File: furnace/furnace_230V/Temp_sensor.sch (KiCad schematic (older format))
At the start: 1 part

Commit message: Add files via upload
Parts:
- added C?: 0,1, Capacitor_SMD:C_0603_1608Metric_Pad1.08x0.95mm_HandSolder, symbol Device:C
- added R?: 4,7k, Resistor_SMD:R_0603_1608Metric_Pad0.98x0.95mm_HandSolder, symbol Device:R
- added TP?: TestPoint, symbol Connector:TestPoint
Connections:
- net labels added: +3V3, GND, SDA
- wire segments 0 -> 14
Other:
- note added: "1-wire temperature sensor"
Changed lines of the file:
@@
 L Sensor_Temperature:DS18B20 U?
 U 1 1 60AB486E
-P 5950 3550
-F 0 "U?" H 5720 3596 50  0000 R CNN
-F 1 "DS18B20" H 5720 3505 50  0000 R CNN
-F 2 "Package_TO_SOT_THT:TO-92_Inline" H 4950 3300 50  0001 C CNN
-F 3 "http://datasheets.maximintegrated.com/en/ds/DS18B20.pdf" H 5800 3800 50  0001 C CNN
-	1    5950 3550
+P 5500 4300
+F 0 "U?" H 5850 4650 50  0000 R CNN
+F 1 "DS18B20" H 6000 4550 50  0000 R CNN
+F 2 "Package_TO_SOT_THT:TO-92_Inline" H 4500 4050 50  0001 C CNN
+F 3 "http://datasheets.maximintegrated.com/en/ds/DS18B20.pdf" H 5350 4550 50  0001 C CNN
+	1    5500 4300
 	1    0    0    -1
 $EndComp
+$Comp
+L Device:C C?
+U 1 1 60AC6956
+P 5000 3650
+AR Path="/60AC6956" Ref="C?"  Part="1"
+AR Path="/609CA6A8/609D24C0/60AC6956" Ref="C?"  Part="1"
+AR Path="/609CA6A8/60A08E0B/60AC6956" Ref="C?"  Part="1"
+AR Path="/609CA6A8/60A0A46E/60AC6956" Ref="C?"  Part="1"
+AR Path="/609CA6A8/60A0A500/60AC6956" Ref="C?"  Part="1"
+AR Path="/609CA6A8/60A0A922/60AC6956" Ref="C?"  Part="1"
+AR Path="/609CA6A8/60AC6956" Ref="C?"  Part="1"
+AR Path="/609CA6A8/60AE5653/60AC6956" Ref="C?"  Part="1"
+AR Path="/60AAC605/60AC6956" Ref="C?"  Part="1"
+AR Path="/60AAE178/60AC6956" Ref="C?"  Part="1"
+F 0 "C?" H 5115 3696 50  0000 L CNN
+F 1 "0,1" H 5115 3605 50  0000 L CNN
+F 2 "Capacitor_SMD:C_0603_1608Metric_Pad1.08x0.95mm_HandSolder" H 5038 3500 50  0001 C CNN
+F 3 "~" H 5000 3650 50  0001 C CNN
+	1    5000 3650
+	1    0    0    -1
+$EndComp
+$Comp
+L Device:R R?
+U 1 1 60AC70EB
+P 6500 3650
+AR Path="/60AC70EB" Ref="R?"  Part="1"
+AR Path="/609CA6A8/60AC70EB" Ref="R?"  Part="1"
+AR Path="/609CA6A8/60AE5653/60AC70EB" Ref="R?"  Part="1"
+AR Path="/60AAC605/60AC70EB" Ref="R?"  Part="1"
+AR Path="/60AAE178/60AC70EB" Ref="R?"  Part="1"
+F 0 "R?" H 6570 3696 50  0000 L CNN
+F 1 "4,7k" H 6570 3605 50  0000 L CNN
+F 2 "Resistor_SMD:R_0603_1608Metric_Pad0.98x0.95mm_HandSolder" V 6430 3650 50  0001 C CNN
+F 3 "~" H 6500 3650 50  0001 C CNN
+	1    6500 3650
+	1    0    0    -1
+$EndComp
+$Comp
+L Connector:TestPoint TP?
+U 1 1 60ACF1AA
+P 7000 4500
+AR Path="/60ACF1AA" Ref="TP?"  Part="1"
+AR Path="/609CA6A8/60AE5653/60ACF1AA" Ref="TP?"  Part="1"
+AR Path="/60AAC605/60ACF1AA" Ref="TP?"  Part="1"
+AR Path="/60AAE178/60ACF1AA" Ref="TP?"  Part="1"
+F 0 "TP?" H 7058 4618 50  0000 L CNN
+F 1 "TestPoint" H 7058 4527 50  0001 L CNN
+F 2 "" H 7200 4500 50  0001 C CNN
+F 3 "~" H 7200 4500 50  0001 C CNN
+	1    7000 4500
+	1    0    0    -1
+$EndComp
+Text Notes 7950 2300 2    197  ~ 0
+1-wire temperature sensor
+Text HLabel 7500 4500 2    50   BiDi ~ 0
+SDA
+Text HLabel 4500 3500 0    50   Input ~ 0
++3V3
+Text HLabel 4500 5000 0    50   Input ~ 0
+GND
+Wire Wire Line
+	4500 3500 5000 3500
+Connection ~ 5000 3500
+Wire Wire Line
+	5000 3500 5500 3500
+Wire Wire Line
+	5500 4000 5500 3500
+Connection ~ 5500 3500
+Wire Wire Line
+	5500 3500 6500 3500
+Wire Wire Line
+	5000 3800 5000 5000
+Wire Wire Line
+	5000 5000 4500 5000
+Wire Wire Line
+	5500 4600 5500 5000
+Wire Wire Line
+	5500 5000 5000 5000
+Connection ~ 5000 5000
+Wire Wire Line
+	5800 4300 6000 4300
+Wire Wire Line
+	6000 4300 6000 4500
+Wire Wire Line
+	6000 4500 6500 4500
+Connection ~ 7000 4500
+Wire Wire Line
+	7000 4500 7500 4500
+Wire Wire Line
+	6500 3800 6500 4500
+Connection ~ 6500 4500
+Wire Wire Line
+	6500 4500 7000 4500
 $EndSCHEMATC

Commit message: Add files via upload
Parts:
- C14: renamed from C?; symbol Device:C -> furnace_230V-rescue:C-Device
- R9: renamed from R?; symbol Device:R -> furnace_230V-rescue:R-Device
- TP6: renamed from TP?; symbol Connector:TestPoint -> furnace_230V-rescue:TestPoint-Connector
- U4: renamed from U?; symbol Sensor_Temperature:DS18B20 -> furnace_230V-rescue:DS18B20-Sensor_Temperature
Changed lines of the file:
@@
 $EndDescr
 $Comp
-L Sensor_Temperature:DS18B20 U?
+L furnace_230V-rescue:DS18B20-Sensor_Temperature U4
 U 1 1 60AB486E
 P 5500 4300
-F 0 "U?" H 5850 4650 50  0000 R CNN
+F 0 "U4" H 5850 4650 50  0000 R CNN
 F 1 "DS18B20" H 6000 4550 50  0000 R CNN
 F 2 "Package_TO_SOT_THT:TO-92_Inline" H 4500 4050 50  0001 C CNN
@@
 $EndComp
 $Comp
-L Device:C C?
+L furnace_230V-rescue:C-Device C?
 U 1 1 60AC6956
 P 5000 3650
@@
 AR Path="/609CA6A8/60AE5653/60AC6956" Ref="C?"  Part="1"
 AR Path="/60AAC605/60AC6956" Ref="C?"  Part="1"
-AR Path="/60AAE178/60AC6956" Ref="C?"  Part="1"
-F 0 "C?" H 5115 3696 50  0000 L CNN
+AR Path="/60AAE178/60AC6956" Ref="C14"  Part="1"
+F 0 "C14" H 5115 3696 50  0000 L CNN
 F 1 "0,1" H 5115 3605 50  0000 L CNN
 F 2 "Capacitor_SMD:C_0603_1608Metric_Pad1.08x0.95mm_HandSolder" H 5038 3500 50  0001 C CNN
@@
 $EndComp
 $Comp
-L Device:R R?
+L furnace_230V-rescue:R-Device R?
 U 1 1 60AC70EB
 P 6500 3650
@@
 AR Path="/609CA6A8/60AE5653/60AC70EB" Ref="R?"  Part="1"
 AR Path="/60AAC605/60AC70EB" Ref="R?"  Part="1"
-AR Path="/60AAE178/60AC70EB" Ref="R?"  Part="1"
-F 0 "R?" H 6570 3696 50  0000 L CNN
+AR Path="/60AAE178/60AC70EB" Ref="R9"  Part="1"
+F 0 "R9" H 6570 3696 50  0000 L CNN
 F 1 "4,7k" H 6570 3605 50  0000 L CNN
 F 2 "Resistor_SMD:R_0603_1608Metric_Pad0.98x0.95mm_HandSolder" V 6430 3650 50  0001 C CNN
@@
 $EndComp
 $Comp
-L Connector:TestPoint TP?
+L furnace_230V-rescue:TestPoint-Connector TP?
 U 1 1 60ACF1AA
 P 7000 4500
@@
 AR Path="/609CA6A8/60AE5653/60ACF1AA" Ref="TP?"  Part="1"
 AR Path="/60AAC605/60ACF1AA" Ref="TP?"  Part="1"
-AR Path="/60AAE178/60ACF1AA" Ref="TP?"  Part="1"
-F 0 "TP?" H 7058 4618 50  0000 L CNN
+AR Path="/60AAE178/60ACF1AA" Ref="TP6"  Part="1"
+F 0 "TP6" H 7058 4618 50  0000 L CNN
 F 1 "TestPoint" H 7058 4527 50  0001 L CNN
 F 2 "" H 7200 4500 50  0001 C CNN

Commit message: Add files via upload
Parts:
- TP6: footprint (none) -> MountingHole:MountingHole_2.2mm_M2_DIN965_Pad_TopBottom
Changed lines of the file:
@@
 F 0 "TP6" H 7058 4618 50  0000 L CNN
 F 1 "TestPoint" H 7058 4527 50  0001 L CNN
-F 2 "" H 7200 4500 50  0001 C CNN
+F 2 "MountingHole:MountingHole_2.2mm_M2_DIN965_Pad_TopBottom" H 7200 4500 50  0001 C CNN
 F 3 "~" H 7200 4500 50  0001 C CNN
 	1    7000 4500

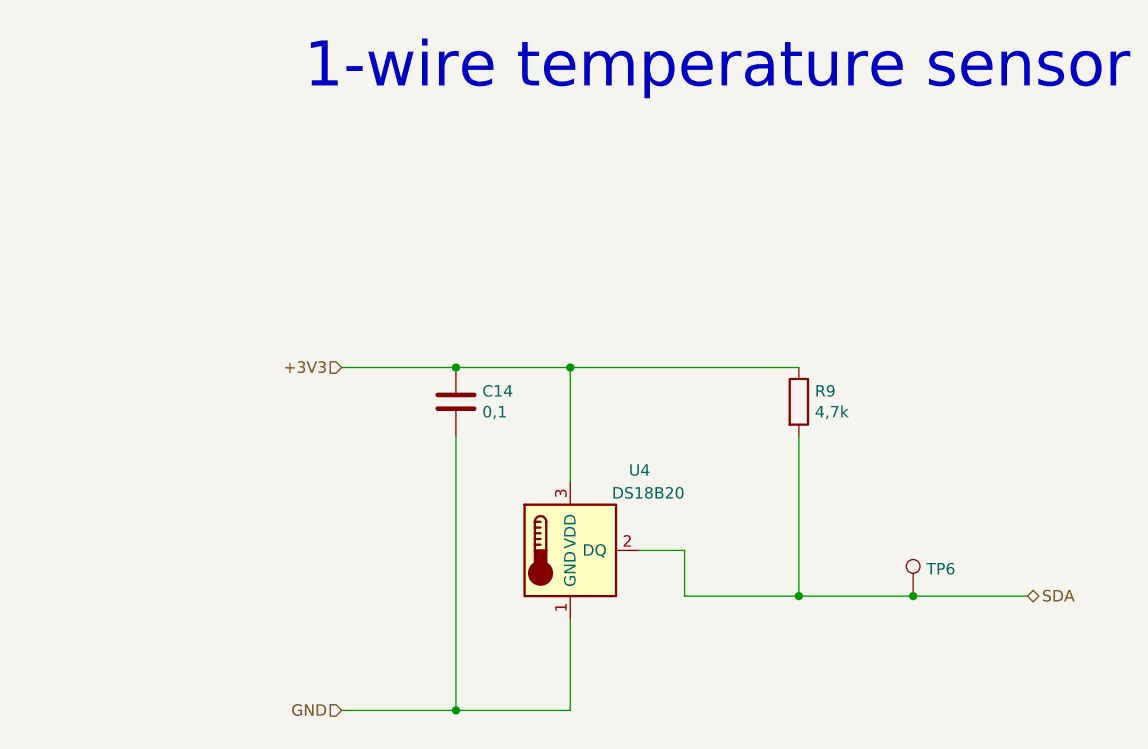
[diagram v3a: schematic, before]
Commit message: Add files via upload
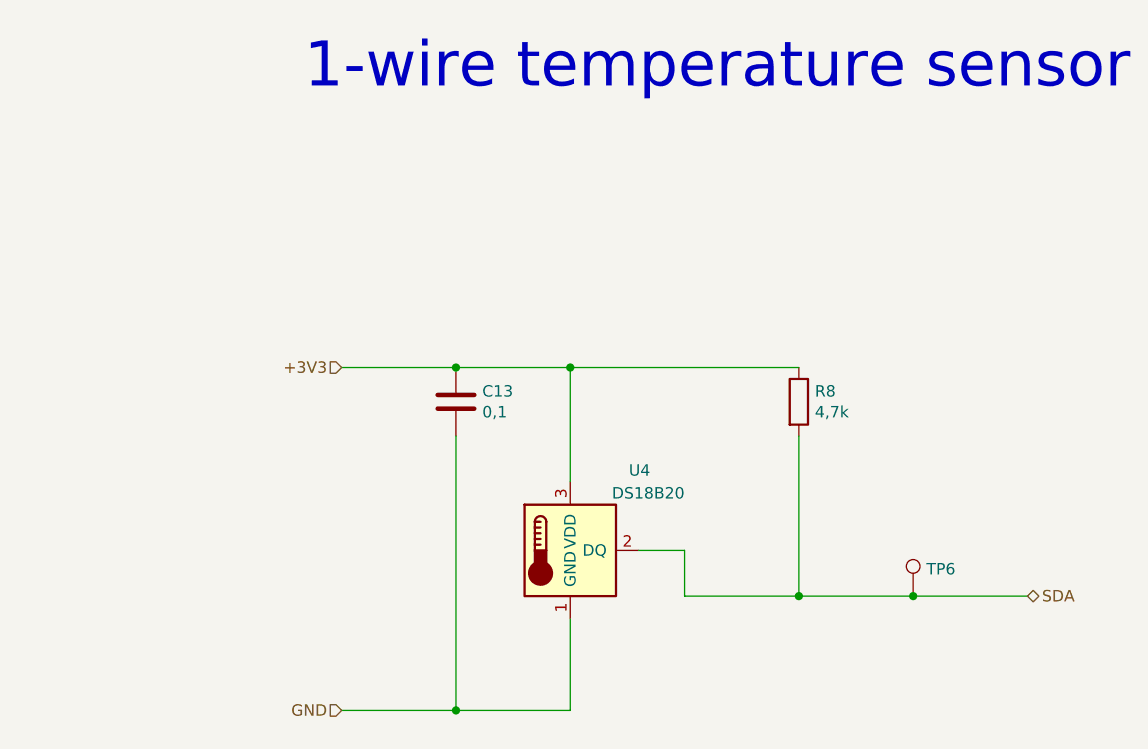
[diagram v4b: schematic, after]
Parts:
- C13: renamed from C14; footprint Capacitor_SMD:C_0603_1608Metric_Pad1.08x0.95mm_HandSolder -> Capacitor_SMD:C_0603_1608Metric_Pad1.05x0.95mm_HandSolder
- R8: renamed from R9; footprint Resistor_SMD:R_0603_1608Metric_Pad0.98x0.95mm_HandSolder -> Resistor_SMD:R_0603_1608Metric_Pad1.05x0.95mm_HandSolder
- TP6: footprint MountingHole:MountingHole_2.2mm_M2_DIN965_Pad_TopBottom -> furnace_230V:TP
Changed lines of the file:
@@
 AR Path="/609CA6A8/60AE5653/60AC6956" Ref="C?"  Part="1"
 AR Path="/60AAC605/60AC6956" Ref="C?"  Part="1"
-AR Path="/60AAE178/60AC6956" Ref="C14"  Part="1"
-F 0 "C14" H 5115 3696 50  0000 L CNN
+AR Path="/60AAE178/60AC6956" Ref="C13"  Part="1"
+F 0 "C13" H 5115 3696 50  0000 L CNN
 F 1 "0,1" H 5115 3605 50  0000 L CNN
-F 2 "Capacitor_SMD:C_0603_1608Metric_Pad1.08x0.95mm_HandSolder" H 5038 3500 50  0001 C CNN
+F 2 "Capacitor_SMD:C_0603_1608Metric_Pad1.05x0.95mm_HandSolder" H 5038 3500 50  0001 C CNN
 F 3 "~" H 5000 3650 50  0001 C CNN
 	1    5000 3650
@@
 AR Path="/609CA6A8/60AE5653/60AC70EB" Ref="R?"  Part="1"
 AR Path="/60AAC605/60AC70EB" Ref="R?"  Part="1"
-AR Path="/60AAE178/60AC70EB" Ref="R9"  Part="1"
-F 0 "R9" H 6570 3696 50  0000 L CNN
+AR Path="/60AAE178/60AC70EB" Ref="R8"  Part="1"
+F 0 "R8" H 6570 3696 50  0000 L CNN
 F 1 "4,7k" H 6570 3605 50  0000 L CNN
-F 2 "Resistor_SMD:R_0603_1608Metric_Pad0.98x0.95mm_HandSolder" V 6430 3650 50  0001 C CNN
+F 2 "Resistor_SMD:R_0603_1608Metric_Pad1.05x0.95mm_HandSolder" V 6430 3650 50  0001 C CNN
 F 3 "~" H 6500 3650 50  0001 C CNN
 	1    6500 3650
@@
 F 0 "TP6" H 7058 4618 50  0000 L CNN
 F 1 "TestPoint" H 7058 4527 50  0001 L CNN
-F 2 "MountingHole:MountingHole_2.2mm_M2_DIN965_Pad_TopBottom" H 7200 4500 50  0001 C CNN
+F 2 "furnace_230V:TP" H 7200 4500 50  0001 C CNN
 F 3 "~" H 7200 4500 50  0001 C CNN
 	1    7000 4500

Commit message: Add files via upload
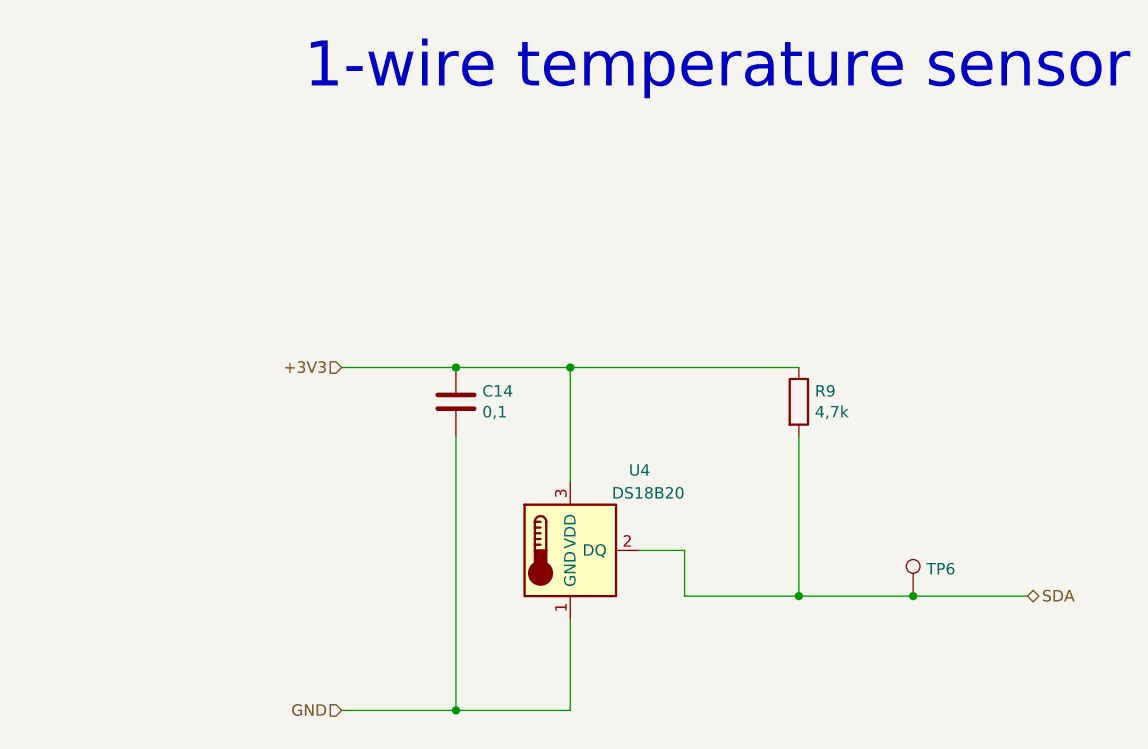
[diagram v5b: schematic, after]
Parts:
- C14: renamed from C13; footprint Capacitor_SMD:C_0603_1608Metric_Pad1.05x0.95mm_HandSolder -> Capacitor_SMD:C_0603_1608Metric_Pad1.08x0.95mm_HandSolder
- R9: renamed from R8; footprint Resistor_SMD:R_0603_1608Metric_Pad1.05x0.95mm_HandSolder -> Resistor_SMD:R_0603_1608Metric_Pad0.98x0.95mm_HandSolder
- TP6: footprint furnace_230V:TP -> MountingHole:MountingHole_2.2mm_M2_DIN965_Pad_TopBottom
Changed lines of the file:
@@
 AR Path="/609CA6A8/60AE5653/60AC6956" Ref="C?"  Part="1"
 AR Path="/60AAC605/60AC6956" Ref="C?"  Part="1"
-AR Path="/60AAE178/60AC6956" Ref="C13"  Part="1"
-F 0 "C13" H 5115 3696 50  0000 L CNN
+AR Path="/60AAE178/60AC6956" Ref="C14"  Part="1"
+F 0 "C14" H 5115 3696 50  0000 L CNN
 F 1 "0,1" H 5115 3605 50  0000 L CNN
-F 2 "Capacitor_SMD:C_0603_1608Metric_Pad1.05x0.95mm_HandSolder" H 5038 3500 50  0001 C CNN
+F 2 "Capacitor_SMD:C_0603_1608Metric_Pad1.08x0.95mm_HandSolder" H 5038 3500 50  0001 C CNN
 F 3 "~" H 5000 3650 50  0001 C CNN
 	1    5000 3650
@@
 AR Path="/609CA6A8/60AE5653/60AC70EB" Ref="R?"  Part="1"
 AR Path="/60AAC605/60AC70EB" Ref="R?"  Part="1"
-AR Path="/60AAE178/60AC70EB" Ref="R8"  Part="1"
-F 0 "R8" H 6570 3696 50  0000 L CNN
+AR Path="/60AAE178/60AC70EB" Ref="R9"  Part="1"
+F 0 "R9" H 6570 3696 50  0000 L CNN
 F 1 "4,7k" H 6570 3605 50  0000 L CNN
-F 2 "Resistor_SMD:R_0603_1608Metric_Pad1.05x0.95mm_HandSolder" V 6430 3650 50  0001 C CNN
+F 2 "Resistor_SMD:R_0603_1608Metric_Pad0.98x0.95mm_HandSolder" V 6430 3650 50  0001 C CNN
 F 3 "~" H 6500 3650 50  0001 C CNN
 	1    6500 3650
@@
 F 0 "TP6" H 7058 4618 50  0000 L CNN
 F 1 "TestPoint" H 7058 4527 50  0001 L CNN
-F 2 "furnace_230V:TP" H 7200 4500 50  0001 C CNN
+F 2 "MountingHole:MountingHole_2.2mm_M2_DIN965_Pad_TopBottom" H 7200 4500 50  0001 C CNN
 F 3 "~" H 7200 4500 50  0001 C CNN
 	1    7000 4500
